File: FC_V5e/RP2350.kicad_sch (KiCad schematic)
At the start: 34 parts, among them U11 W25Q128JVS, U18 RP2350_60QFN, U5 APS1604M-3SQR-SN_C18214056, Y1 ABM8-272-T3

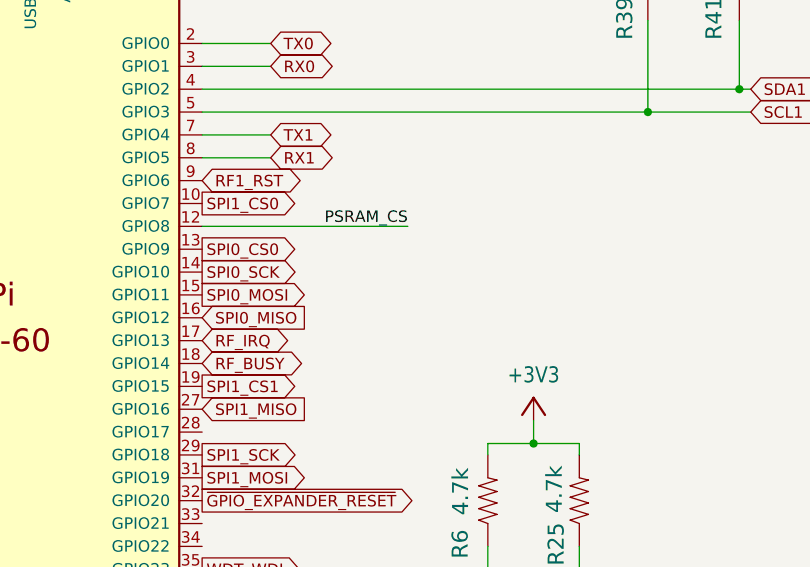
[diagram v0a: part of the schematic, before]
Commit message: Fixed Vias?
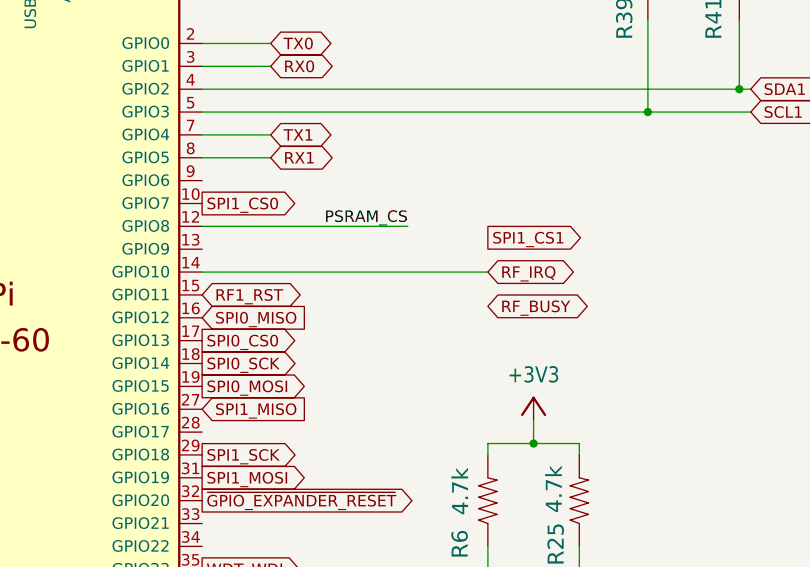
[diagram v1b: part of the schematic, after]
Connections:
- net RF1_RST: now also U18.15 (GPIO11); no longer U18.9 (GPIO6)
- net RF_BUSY: no longer U18.18 (GPIO14)
- net RF_IRQ: now also U18.14 (GPIO10); no longer U18.17 (GPIO13)
- net SPI0_CS0: now also U18.17 (GPIO13); no longer U18.13 (GPIO9)
- net SPI0_MOSI: now also U18.19 (GPIO15); no longer U18.15 (GPIO11)
- net SPI0_SCK: now also U18.18 (GPIO14); no longer U18.14 (GPIO10)
- net SPI1_CS1: no longer U18.19 (GPIO15)
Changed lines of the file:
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@@
+	(wire
+		(pts
+			(xy 241.3 97.79) (xy 209.55 97.79)
+		)
+		(stroke
+			(width 0)
+			(type default)
+		)
+	)
 	(wire
 		(pts
@@
 		)
 	)
+	(global_label "RF1_RST"
+		(shape bidirectional)
+		(at 209.55 100.33 0)
+		(fields_autoplaced yes)
+		(effects
+			(font
+				(size 1.27 1.27)
+			)
+			(justify left)
+		)
+		(property "Intersheetrefs" "${INTERSHEET_REFS}"
+			(at 219.946 100.4094 0)
+			(effects
+				(font
+					(size 1.27 1.27)
+				)
+				(justify left)
+				(hide yes)
+			)
+		)
+	)
+	(global_label "RF_BUSY"
+		(shape bidirectional)
+		(at 241.3 101.6 0)
+		(fields_autoplaced yes)
+		(effects
+			(font
+				(size 1.27 1.27)
+			)
+			(justify left)
+		)
+		(property "Intersheetrefs" "${INTERSHEET_REFS}"
+			(at 253.6213 101.6 0)
+			(effects
+				(font
+					(size 1.27 1.27)
+				)
+				(justify left)
+				(hide yes)
+			)
+		)
+	)
 	(global_label "RTC_INT"
 		(shape input)
@@
 		)
 	)
-	(global_label "RF_IRQ"
-		(shape bidirectional)
-		(at 209.55 105.41 0)
-		(fields_autoplaced yes)
-		(effects
-			(font
-				(size 1.27 1.27)
-			)
-			(justify left)
-		)
-		(property "Intersheetrefs" "${INTERSHEET_REFS}"
-			(at 220.178 105.41 0)
-			(effects
-				(font
-					(size 1.27 1.27)
-				)
-				(justify left)
-				(hide yes)
-			)
-		)
-	)
 	(global_label "FIRE_DEPLOY1_A"
 		(shape output)
@@
 		)
 	)
-	(global_label "SPI1_CS1"
-		(shape output)
-		(at 209.55 110.49 0)
-		(fields_autoplaced yes)
-		(effects
-			(font
-				(size 1.27 1.27)
-			)
-			(justify left)
-		)
-		(property "Intersheetrefs" "${INTERSHEET_REFS}"
-			(at 221.4856 110.49 0)
-			(effects
-				(font
-					(size 1.27 1.27)
-				)
-				(justify left)
-				(hide yes)
-			)
-		)
-	)
 	(global_label "USB_DM"
 		(shape input)
@@
 		)
 	)
+	(global_label "SPI0_CS0"
+		(shape output)
+		(at 209.55 105.41 0)
+		(fields_autoplaced yes)
+		(effects
+			(font
+				(size 1.27 1.27)
+			)
+			(justify left)
+		)
+		(property "Intersheetrefs" "${INTERSHEET_REFS}"
+			(at 221.4062 105.41 0)
+			(effects
+				(font
+					(size 1.27 1.27)
+				)
+				(justify left)
+				(hide yes)
+			)
+		)
+	)
 	(global_label "SWDIO"
 		(shape input)
@@
 		)
 	)
+	(global_label "SPI0_MOSI"
+		(shape output)
+		(at 209.55 110.49 0)
+		(fields_autoplaced yes)
+		(effects
+			(font
+				(size 1.27 1.27)
+			)
+			(justify left)
+		)
+		(property "Intersheetrefs" "${INTERSHEET_REFS}"
+			(at 222.3134 110.49 0)
+			(effects
+				(font
+					(size 1.27 1.27)
+				)
+				(justify left)
+				(hide yes)
+			)
+		)
+	)
 	(global_label "RX0"
 		(shape bidirectional)
@@
 		)
 	)
-	(global_label "RF_BUSY"
-		(shape bidirectional)
-		(at 209.55 107.95 0)
-		(fields_autoplaced yes)
-		(effects
-			(font
-				(size 1.27 1.27)
-			)
-			(justify left)
-		)
-		(property "Intersheetrefs" "${INTERSHEET_REFS}"
-			(at 221.8713 107.95 0)
-			(effects
-				(font
-					(size 1.27 1.27)
-				)
-				(justify left)
-				(hide yes)
-			)
-		)
-	)
 	(global_label "FC_RESET"
 		(shape bidirectional)
@@
 		)
 	)
+	(global_label "RF_IRQ"
+		(shape bidirectional)
+		(at 241.3 97.79 0)
+		(fields_autoplaced yes)
+		(effects
+			(font
+				(size 1.27 1.27)
+			)
+			(justify left)
+		)
+		(property "Intersheetrefs" "${INTERSHEET_REFS}"
+			(at 251.928 97.79 0)
+			(effects
+				(font
+					(size 1.27 1.27)
+				)
+				(justify left)
+				(hide yes)
+			)
+		)
+	)
+	(global_label "SPI1_CS1"
+		(shape output)
+		(at 241.3 93.98 0)
+		(fields_autoplaced yes)
+		(effects
+			(font
+				(size 1.27 1.27)
+			)
+			(justify left)
+		)
+		(property "Intersheetrefs" "${INTERSHEET_REFS}"
+			(at 253.2356 93.98 0)
+			(effects
+				(font
+					(size 1.27 1.27)
+				)
+				(justify left)
+				(hide yes)
+			)
+		)
+	)
 	(global_label "TX0"
 		(shape bidirectional)
@@
 		)
 	)
-	(global_label "SPI0_CS0"
+	(global_label "SPI0_SCK"
 		(shape output)
-		(at 209.55 95.25 0)
-		(fields_autoplaced yes)
-		(effects
-			(font
-				(size 1.27 1.27)
-			)
-			(justify left)
-		)
-		(property "Intersheetrefs" "${INTERSHEET_REFS}"
-			(at 221.4062 95.25 0)
+		(at 209.55 107.95 0)
+		(fields_autoplaced yes)
+		(effects
+			(font
+				(size 1.27 1.27)
+			)
+			(justify left)
+		)
+		(property "Intersheetrefs" "${INTERSHEET_REFS}"
+			(at 221.4667 107.95 0)
 			(effects
 				(font
@@
 		)
 	)
-	(global_label "SPI0_MOSI"
-		(shape output)
-		(at 209.55 100.33 0)
-		(fields_autoplaced yes)
-		(effects
-			(font
-				(size 1.27 1.27)
-			)
-			(justify left)
-		)
-		(property "Intersheetrefs" "${INTERSHEET_REFS}"
-			(at 222.3134 100.33 0)
-			(effects
-				(font
-					(size 1.27 1.27)
-				)
-				(justify left)
-				(hide yes)
-			)
-		)
-	)
 	(global_label "FIRE_DEPLOY1_B"
 		(shape output)
@@
 		)
 	)
-	(global_label "SPI0_SCK"
-		(shape output)
-		(at 209.55 97.79 0)
-		(fields_autoplaced yes)
-		(effects
-			(font
-				(size 1.27 1.27)
-			)
-			(justify left)
-		)
-		(property "Intersheetrefs" "${INTERSHEET_REFS}"
-			(at 221.4667 97.79 0)
-			(effects
-				(font
-					(size 1.27 1.27)
-				)
-				(justify left)
-				(hide yes)
-			)
-		)
-	)
 	(global_label "SPI1_CS0"
 		(shape output)
@@
 			(effects
 				(font
-					(size 1.27 1.27)
-				)
-				(justify left)
-				(hide yes)
-			)
-		)
-	)
-	(global_label "RF1_RST"
-		(shape bidirectional)
-		(at 209.55 87.63 0)
-		(fields_autoplaced yes)
-		(effects
-			(font
-				(size 1.27 1.27)
-			)
-			(justify left)
-		)
-		(property "Intersheetrefs" "${INTERSHEET_REFS}"
-			(at 219.946 87.7094 0)
-			(effects
-				(font

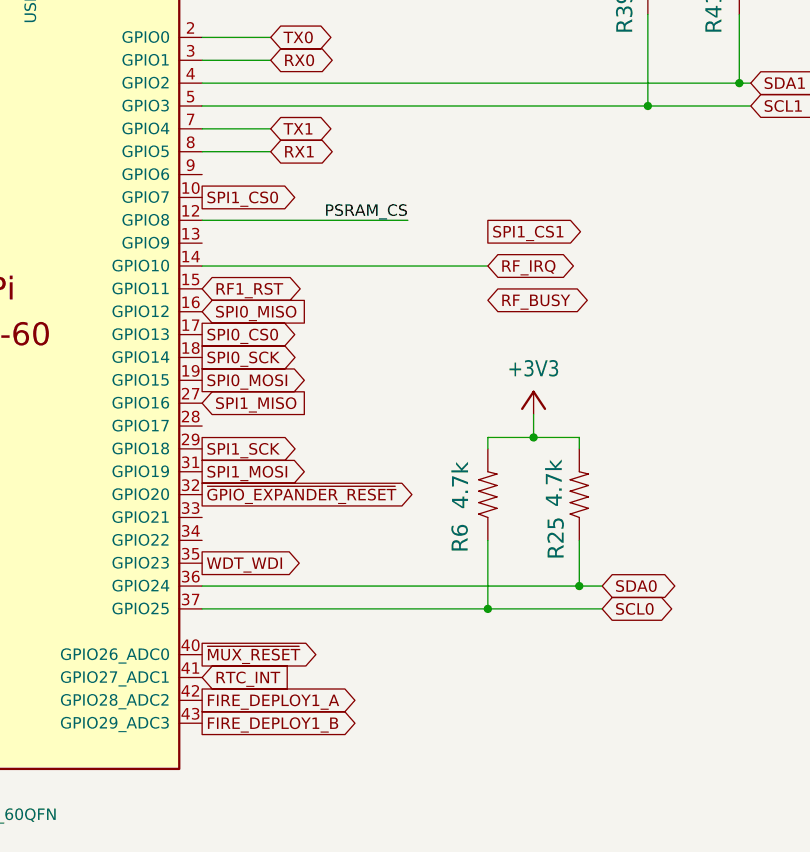
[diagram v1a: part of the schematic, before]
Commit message: Renamed V5d Rev 3 to V5e
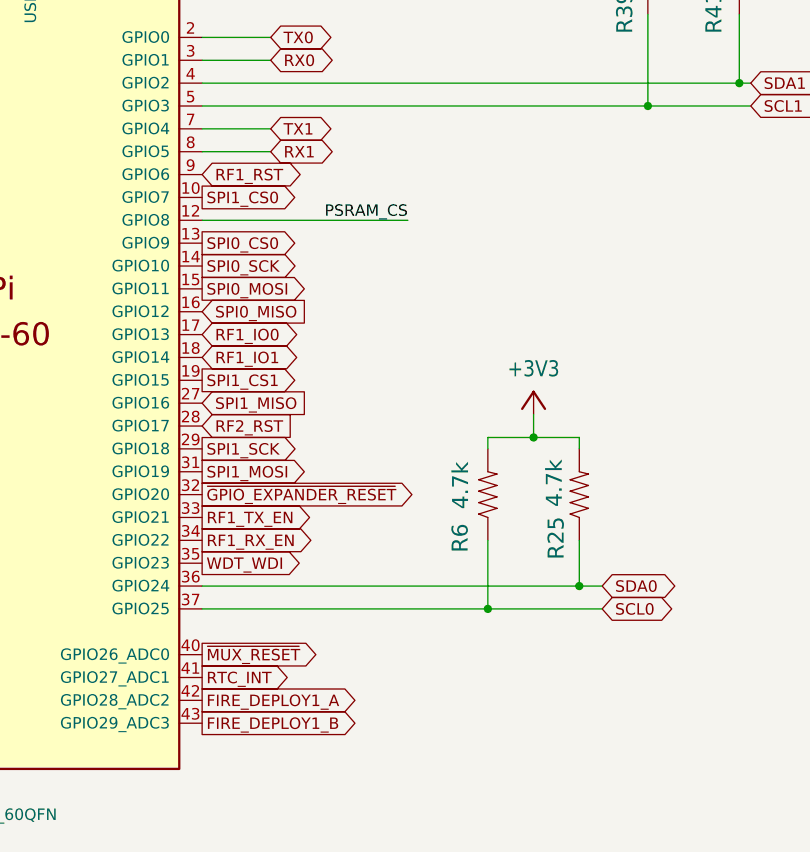
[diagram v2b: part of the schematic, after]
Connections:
- net RF_IRQ is gone; now on net SPI0_SCK: U18.14 (GPIO10)
- net RF1_RST: now also U18.9 (GPIO6); no longer U18.15 (GPIO11)
- net SPI0_CS0: now also U18.13 (GPIO9); no longer U18.17 (GPIO13)
- net SPI0_MOSI: now also U18.15 (GPIO11); no longer U18.19 (GPIO15)
- net SPI0_SCK: no longer U18.18 (GPIO14)
- net SPI1_CS1: now also U18.19 (GPIO15)
- net RF2_RST: now reaches U18.28 (GPIO17)
- net RF1_TX_EN: now reaches U18.33 (GPIO21)
- net RF1_RX_EN: now reaches U18.34 (GPIO22)
- new net RF1_IO0: U18.17 (GPIO13)
- new net RF1_IO1: U18.18 (GPIO14)
